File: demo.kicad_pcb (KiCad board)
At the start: 2 copper layers, 37 x 25 mm, 31 parts, among them J1 download_firmware, J2 USB_B_Micro, J3 stlink_interface, U1 STM32F103C8Tx, U2 AMS1117-3.3, Y1 Crystal

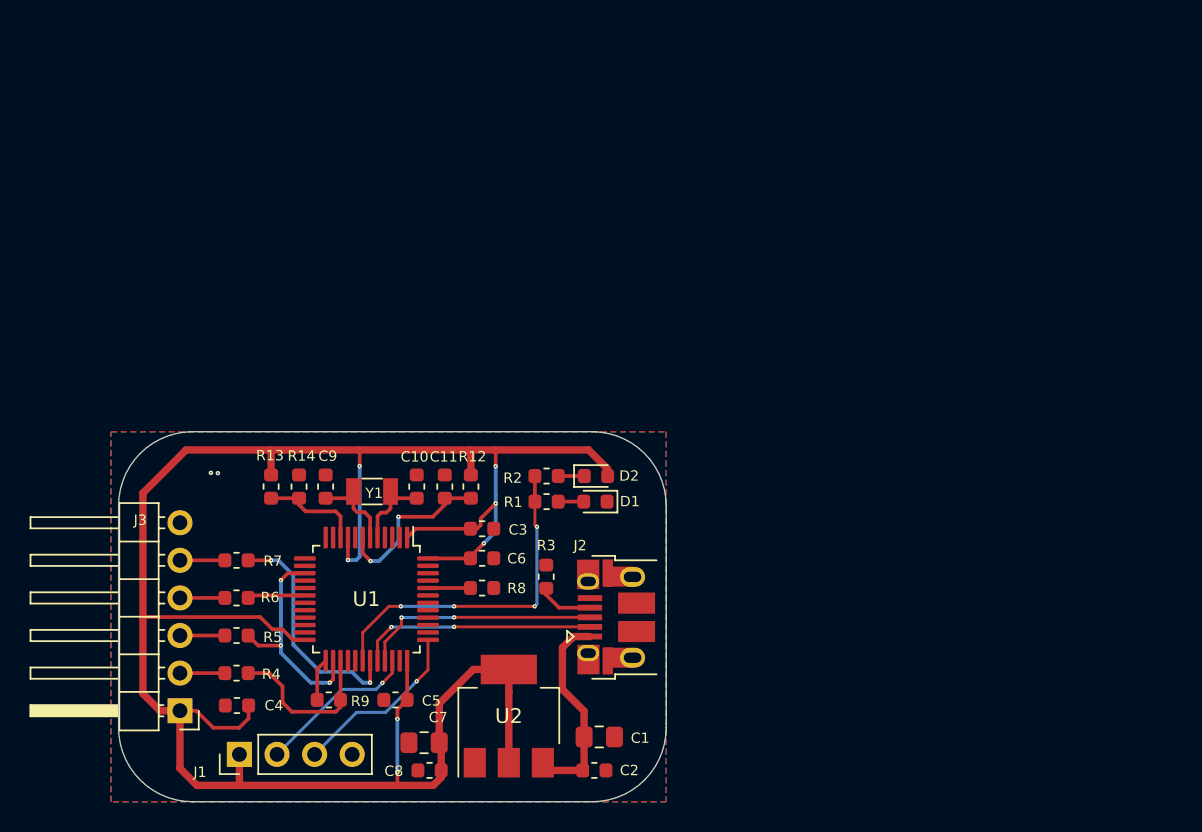
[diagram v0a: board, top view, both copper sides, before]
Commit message: v1.0.0
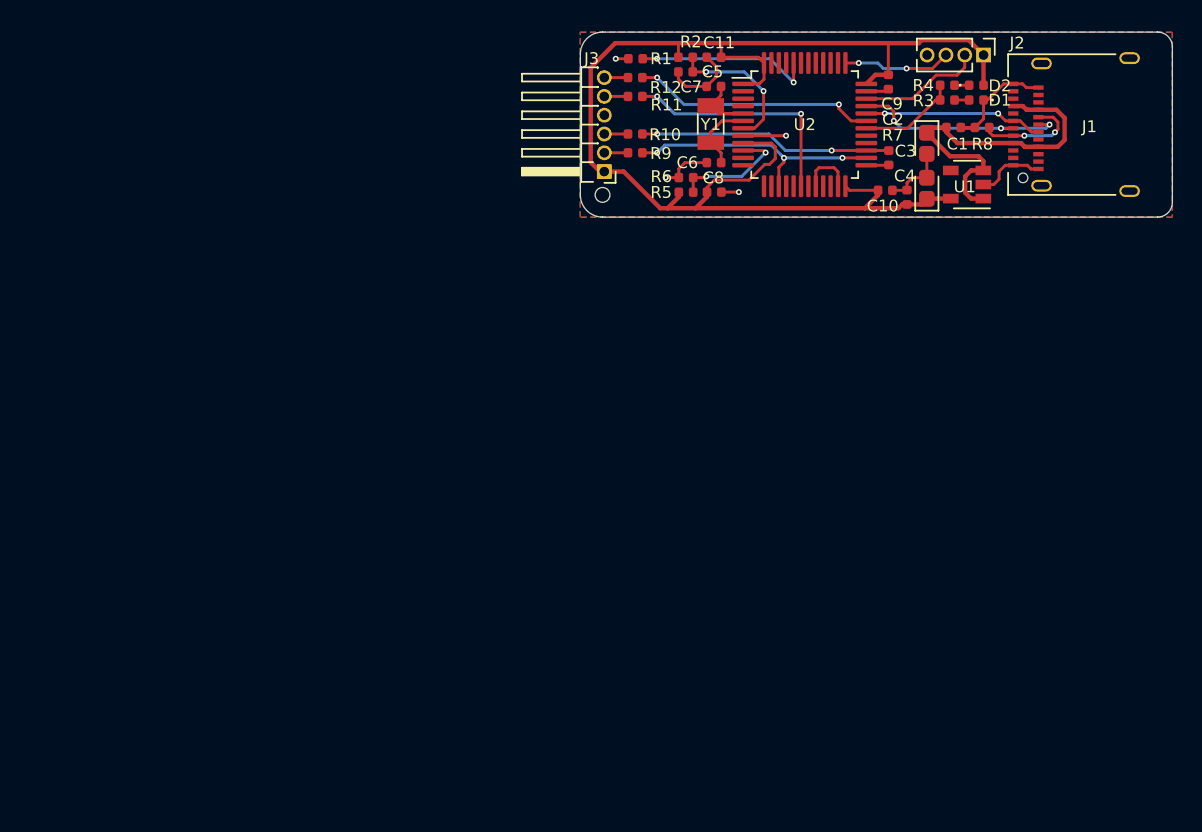
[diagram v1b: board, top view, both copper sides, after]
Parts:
- removed R13, R14: 4K7, hardware-demo:R_0603_1608Metric
- added R10: 22, hardware-demo:R_0402_1005Metric, F.Cu at (98.7, 106.9)
- added R11: 22, hardware-demo:R_0402_1005Metric, F.Cu at (98.7, 104.3)
- added REF**: installHole, hardware-demo:installHole, F.Cu at (96.5, 111.0)
- C1: value 10uF -> 0.1uF; footprint hardware-demo:C_0805_2012Metric_Pad1.15x1.40mm_HandSolder -> hardware-demo:C_0402_1005Metric
- C10, C9: value 10pF -> 100nF; footprint hardware-demo:C_0603_1608Metric -> hardware-demo:C_0402_1005Metric
- C11, C5: footprint hardware-demo:C_0603_1608Metric -> hardware-demo:C_0402_1005Metric
- C2: value 0.1uF -> 10uF; footprint hardware-demo:C_0603_1608Metric -> Capacitor_Tantalum_SMD:CP_EIA-1608-10_AVX-L
- C3: value 100nF -> 10uF; footprint hardware-demo:C_0603_1608Metric -> Capacitor_Tantalum_SMD:CP_EIA-1608-10_AVX-L
- C4: value 100nF -> 0.1uF; footprint hardware-demo:C_0603_1608Metric -> hardware-demo:C_0402_1005Metric
- C6: value 100nF -> 10pF; footprint hardware-demo:C_0603_1608Metric -> hardware-demo:C_0402_1005Metric
- C7: value 10uF -> 10pF; footprint hardware-demo:C_0805_2012Metric_Pad1.15x1.40mm_HandSolder -> hardware-demo:C_0402_1005Metric
- C8: value 0.1uF -> 100nF; footprint hardware-demo:C_0603_1608Metric -> hardware-demo:C_0402_1005Metric
- D1, D2: footprint hardware-demo:LED_0603_1608Metric -> hardware-demo:LED_0402_1005Metric
- J1: value download_firmware -> USB_C_Receptacle_USB2.0; footprint hardware-demo:PinHeader_1x04_P2.54mm_Vertical -> hardware-demo:USB_C_Receptacle_Amphenol_12401610E4-2A
- J2: value USB_B_Micro -> download_firmware; footprint hardware-demo:USB_Micro-B_Amphenol_10103594-0001LF_Horizontal -> Connector_PinHeader_1.27mm:PinHeader_1x04_P1.27mm_Vertical
- J3: footprint hardware-demo:PinHeader_1x06_P2.54mm_Horizontal -> hardware-demo:PinHeader_1x06_P1.27mm_Horizontal
- R1, R2: value 100R -> 100K; footprint hardware-demo:R_0603_1608Metric -> hardware-demo:R_0402_1005Metric
- R12: value 100K -> 22; footprint hardware-demo:R_0603_1608Metric -> hardware-demo:R_0402_1005Metric
- R3: value 100K -> 100R; footprint hardware-demo:R_0603_1608Metric -> hardware-demo:R_0402_1005Metric
- R4, R7: value 22 -> 100R; footprint hardware-demo:R_0603_1608Metric -> hardware-demo:R_0402_1005Metric
- R5, R6: value 22 -> 4K7; footprint hardware-demo:R_0603_1608Metric -> hardware-demo:R_0402_1005Metric
- R8: value 100K -> 5K1; footprint hardware-demo:R_0603_1608Metric -> hardware-demo:R_0402_1005Metric
- R9: value 100R -> 22; footprint hardware-demo:R_0603_1608Metric -> hardware-demo:R_0402_1005Metric
- U1: value STM32F103C8Tx -> XC6220B331MR; footprint hardware-demo:LQFP-48_7x7mm_P0.5mm -> hardware-demo:SOT-23-5
- U2: value AMS1117-3.3 -> STM32F103C8Tx; footprint hardware-demo:SOT-223-3_TabPin2 -> hardware-demo:LQFP-48_7x7mm_P0.5mm
- moved J1 71.4 mm to (129.3, 106.2)
- moved R4 62.3 mm to (119.8, 103.6)
- moved C4 56.8 mm to (117.1, 111.2), turned to 90 degrees
- moved R7 51.8 mm to (115.8, 108.5), turned to 90 degrees
- moved U1 49.3 mm to (121.1, 110.3), turned to 180 degrees
- moved C7 48.5 mm to (104.0, 103.7), turned to 0 degrees
- moved C2 48.0 mm to (118.4, 107.5), turned to 270 degrees
- moved C1 47.6 mm to (120.2, 106.4)
- moved C9 46.8 mm to (115.8, 103.4)
- moved C5 46.7 mm to (102.1, 102.7)
- moved J3 46.4 mm to (96.6, 109.4)
- moved R8 45.9 mm to (122.1, 106.4)
- moved J2 45.4 mm to (122.2, 101.5), turned to 270 degrees
- moved U2 44.7 mm to (110.2, 106.2), turned to 0 degrees
- moved C8 43.5 mm to (104.0, 110.8), turned to 0 degrees
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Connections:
- C10 pad 1: GND -> +3V3
- C10 pad 2: Net-(C10-Pad2) -> GND
- C11 pad 1: /NRST -> +3V3
- C5 pad 1: +3V3 -> /NRST
- C6 pad 1: +3V3 -> GND
- C6 pad 2: GND -> Net-(C6-Pad2)
- C7 pad 1: +3V3 -> GND
- C7 pad 2: GND -> Net-(C7-Pad2)
- C9 pad 1: GND -> +3V3
- C9 pad 2: Net-(C9-Pad2) -> GND
- J2 pad 1: +5V -> +3V3
- J2 pad 2: /STLINK_USB_DM- -> /STM_JTMS
- J2 pad 3: /STLINK_USB_DP+ -> /STM_JTCK
- J2 pad 4: Net-(J2-Pad4) -> GND
- J3 pad 2: /SWDIO -> /SWCLK
- J3 pad 3: /SWCLK -> /SWDIO
- J3 pad 4: Net-(J3-Pad4) -> GND
- J3 pad 6: GND -> Net-(J3-Pad6)
- R1 pad 1: Net-(D1-Pad2) -> /BOOT0
- R1 pad 2: /LED_STLINK -> GND
- R12 pad 1: +3V3 -> /SWO
- R12 pad 2: /NRST -> Net-(J3-Pad6)
- R2 pad 1: Net-(D2-Pad1) -> +3V3
- R2 pad 2: /LED_STLINK -> /NRST
- R3 pad 1: GND -> Net-(D1-Pad2)
- R3 pad 2: Net-(J2-Pad4) -> /LED_STLINK
- R4 pad 1: /T_JTMS -> Net-(D2-Pad1)
- R4 pad 2: /SWDIO -> /LED_STLINK
- R5 pad 1: /T_JTCK -> Net-(R5-Pad1)
- R5 pad 2: /SWCLK -> +3V3
- R6 pad 1: /T_NRST -> GND
- R6 pad 2: Net-(J3-Pad4) -> Net-(R5-Pad1)
- R7 pad 1: /SWO -> /T_SWDIO_IN
- R7 pad 2: Net-(J3-Pad5) -> /T_JTMS
- R8 pad 1: /BOOT0 -> GND
- R8 pad 2: GND -> Net-(J1-PadA5)
- R9 pad 1: /T_SWDIO_IN -> /T_JTCK
- R9 pad 2: /T_JTMS -> /SWCLK
- U1 pad 1: +3V3 -> +5V
- U1 pad 2: (no net) -> GND
- U1 pad 3: (no net) -> +5V
- U1 pad 5: Net-(C10-Pad2) -> +3V3
- U2 pad 1: GND -> +3V3
- U2 pad 2: +3V3 -> (no net)
- U2 pad 3: +5V -> (no net)
- Y1 pad 1: Net-(C9-Pad2) -> Net-(C6-Pad2)
- Y1 pad 2: Net-(C10-Pad2) -> Net-(C7-Pad2)
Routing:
- net +3V3: track 150.3 -> 89.8 mm, vias 7 -> 0
- net GND: track 0.00 -> 35.4 mm, vias 2 -> 4
- net /LED_STLINK: track 23.2 -> 6.78 mm, vias 4 -> 0
- net /T_NRST: track 3.89 -> 16.1 mm, vias 0 -> 2
- net +5V: track 14.0 -> 24.8 mm
- net /BOOT0: track 2.87 -> 12.2 mm, vias 0 -> 2
- net Net-(R5-Pad1): track 0.00 -> 8.17 mm, vias 0 -> 2
- net Net-(J1-PadA5): track 0.00 -> 7.30 mm, vias 0 -> 2
- net Net-(R13-Pad1): track 6.89 -> 0.00 mm
- net Net-(C9-Pad2): track 5.94 -> 0.00 mm
- net /T_JTMS: track 11.2 -> 17.1 mm, vias 0 -> 2
- net Net-(C10-Pad2): track 5.65 -> 0.00 mm
- net Net-(C6-Pad2): track 0.00 -> 4.85 mm
- net /STM_JTCK: track 12.1 -> 7.32 mm, vias 1 -> 2
- net Net-(C7-Pad2): track 0.00 -> 3.99 mm
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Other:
- board size 37 x 25 mm -> 40 x 12.5 mm
- net class Default: trace_width 0.25 -> 0.2
- net class power-3v3: trace_width 0.5 -> 0.3; via_dia 1 -> 0.8; via_drill 0.5 -> 0.4
- rule via_min_drill: 0.3 -> 0.2
- board text added: "3V3"
- board text added: "GND"
- board text added: "NRST"
- board text added: "SWCLK"
- board text added: "SWDIO"
- board text added: "SWO"
- board text added: "designed by wangzefeng"
- board text added: "https://github.com/ZefengWang/hardware-demo"
- board text added: "wangzefeng9@foxmail.com"
